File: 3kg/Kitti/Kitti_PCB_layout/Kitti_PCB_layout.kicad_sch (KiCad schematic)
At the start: 39 parts, among them IC1 TEENSY_4.1, J1 JS17250, J10 Omron E3Z-D82, J11 Omron E3Z-D82, J12 Omron E3Z-D82, J13 Omron E3Z-D82, J14 Omron E3Z-D82, J15 Omron E3Z-D82, J16 Omron E3Z-D82, J17 Omron E3Z-D82, J18 Conn_02x05_Odd_Even, J19 Conn_01x03_Pin, J2 JS17250, J3 JS17250, J4 JS17250, J5 TF_mini, J6 TF_mini, J7 TF_mini, J8 TF_mini, J9 Omron E3Z-D82, U1 AMS1117-5.0

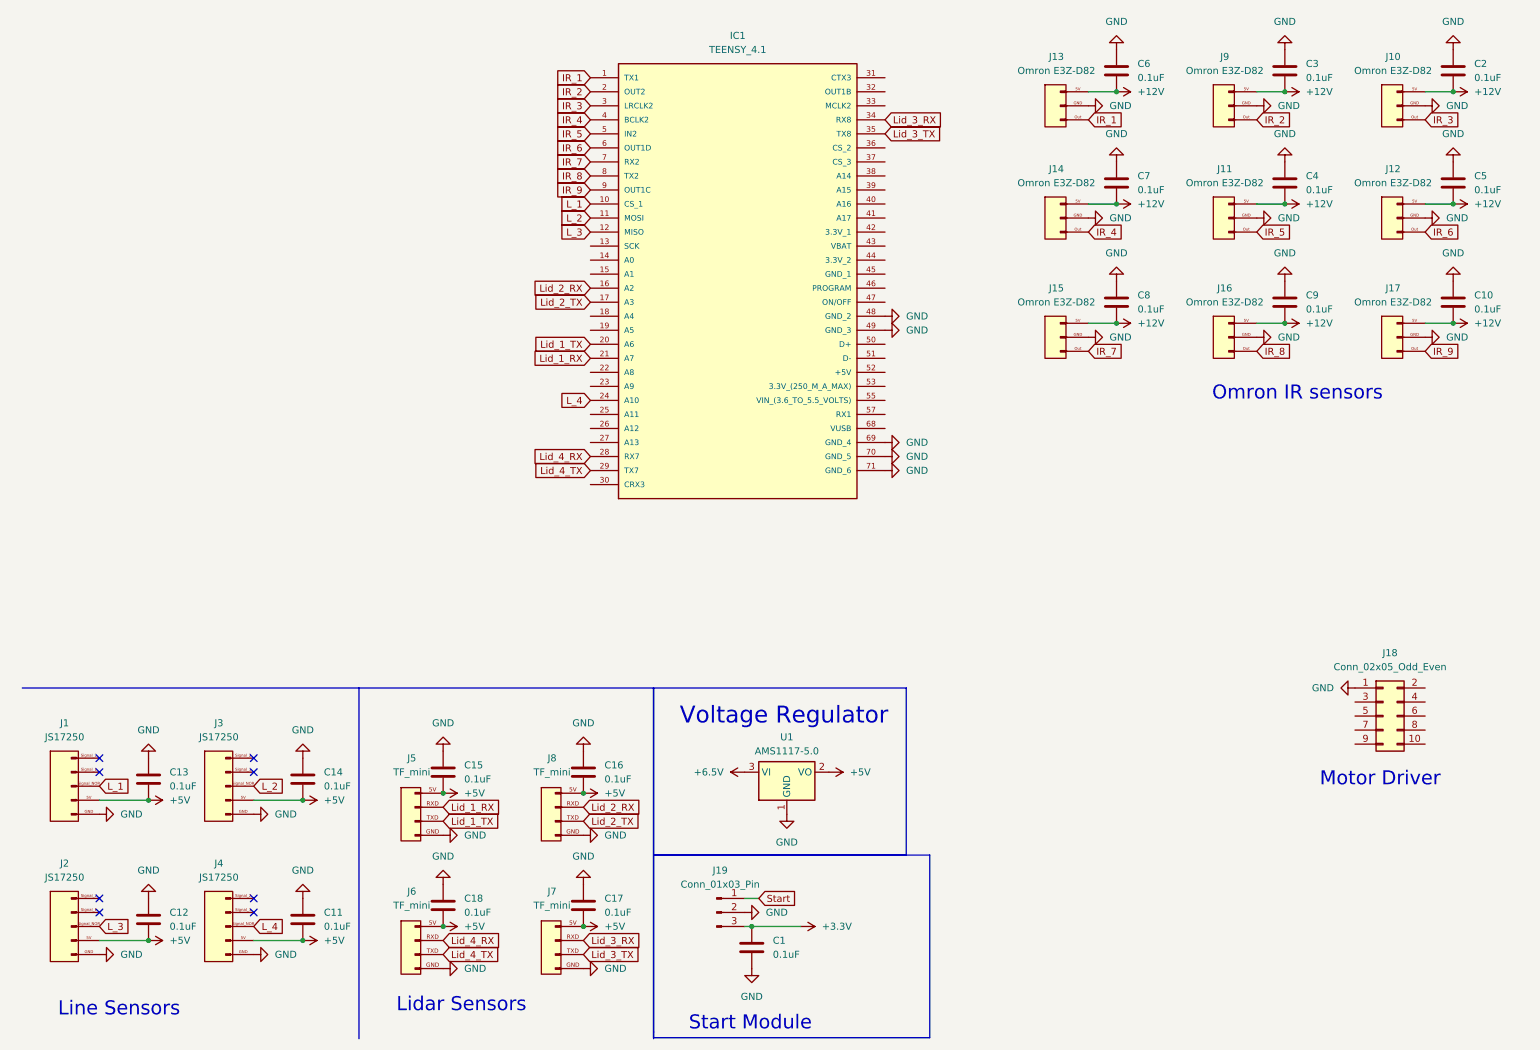
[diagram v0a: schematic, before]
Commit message: resistor and motor driver
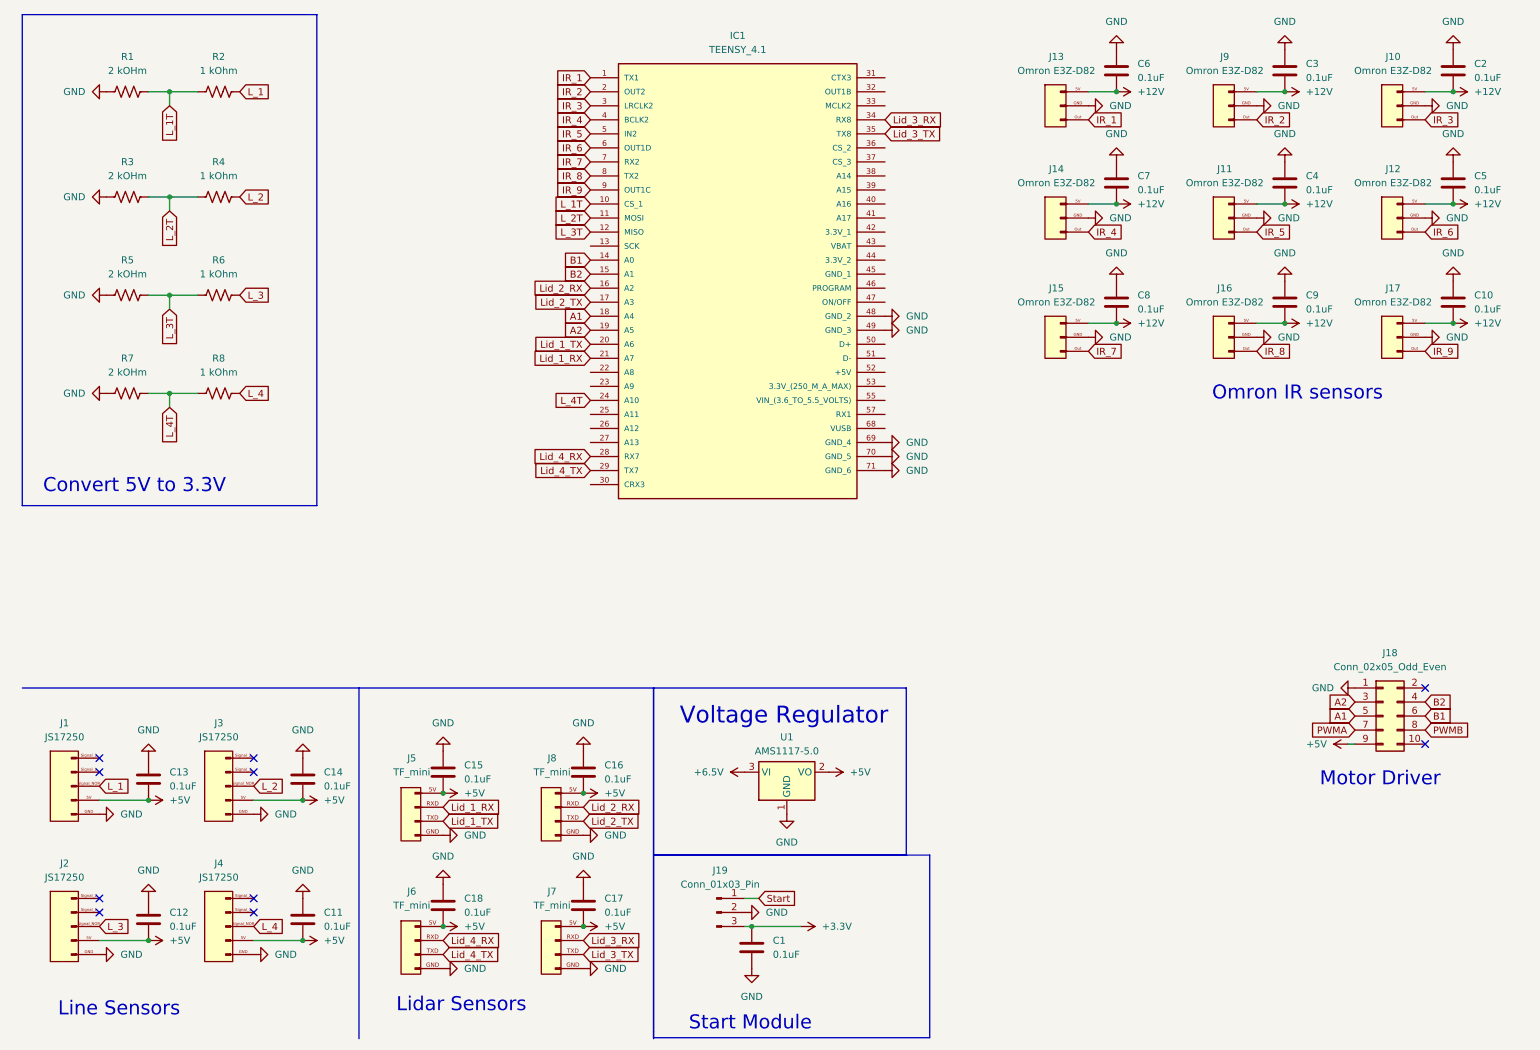
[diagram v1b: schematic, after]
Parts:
- added R1, R3, R5, R7: 2 kOHm, symbol Device:R_US
- added R2, R4, R6, R8: 1 kOhm, symbol Device:R_US
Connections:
- net +5V: now also J18.9 (Pin_9)
- net GND: now also R1.1, R3.1, R5.1, R7.1
- net L_1: now also R2.2; no longer IC1.10 (CS_1)
- net L_2: now also R4.2; no longer IC1.11 (MOSI)
- net L_3: now also R6.2; no longer IC1.12 (MISO)
- net L_4: now also R8.2; no longer IC1.24 (A10)
- net A2: now reaches J18.3 (Pin_3)
- net A2: now also IC1.19 (A5)
- net B2: now reaches J18.4 (Pin_4)
- net B2: now also IC1.15 (A1)
- net A1: now reaches J18.5 (Pin_5)
- net A1: now also IC1.18 (A4)
- net B1: now reaches J18.6 (Pin_6)
- net B1: now also IC1.14 (A0)
- net PWMA: now reaches J18.7 (Pin_7)
- net PWMB: now reaches J18.8 (Pin_8)
- new net L_1T: IC1.10 (CS_1), R1.2, R2.1
- new net L_2T: IC1.11 (MOSI), R3.2, R4.1
- new net L_3T: IC1.12 (MISO), R5.2, R6.1
- new net L_4T: IC1.24 (A10), R7.2, R8.1
- no-connect marks 8 -> 10
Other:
- note added: "Convert 5V to 3.3V"

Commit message: kitti
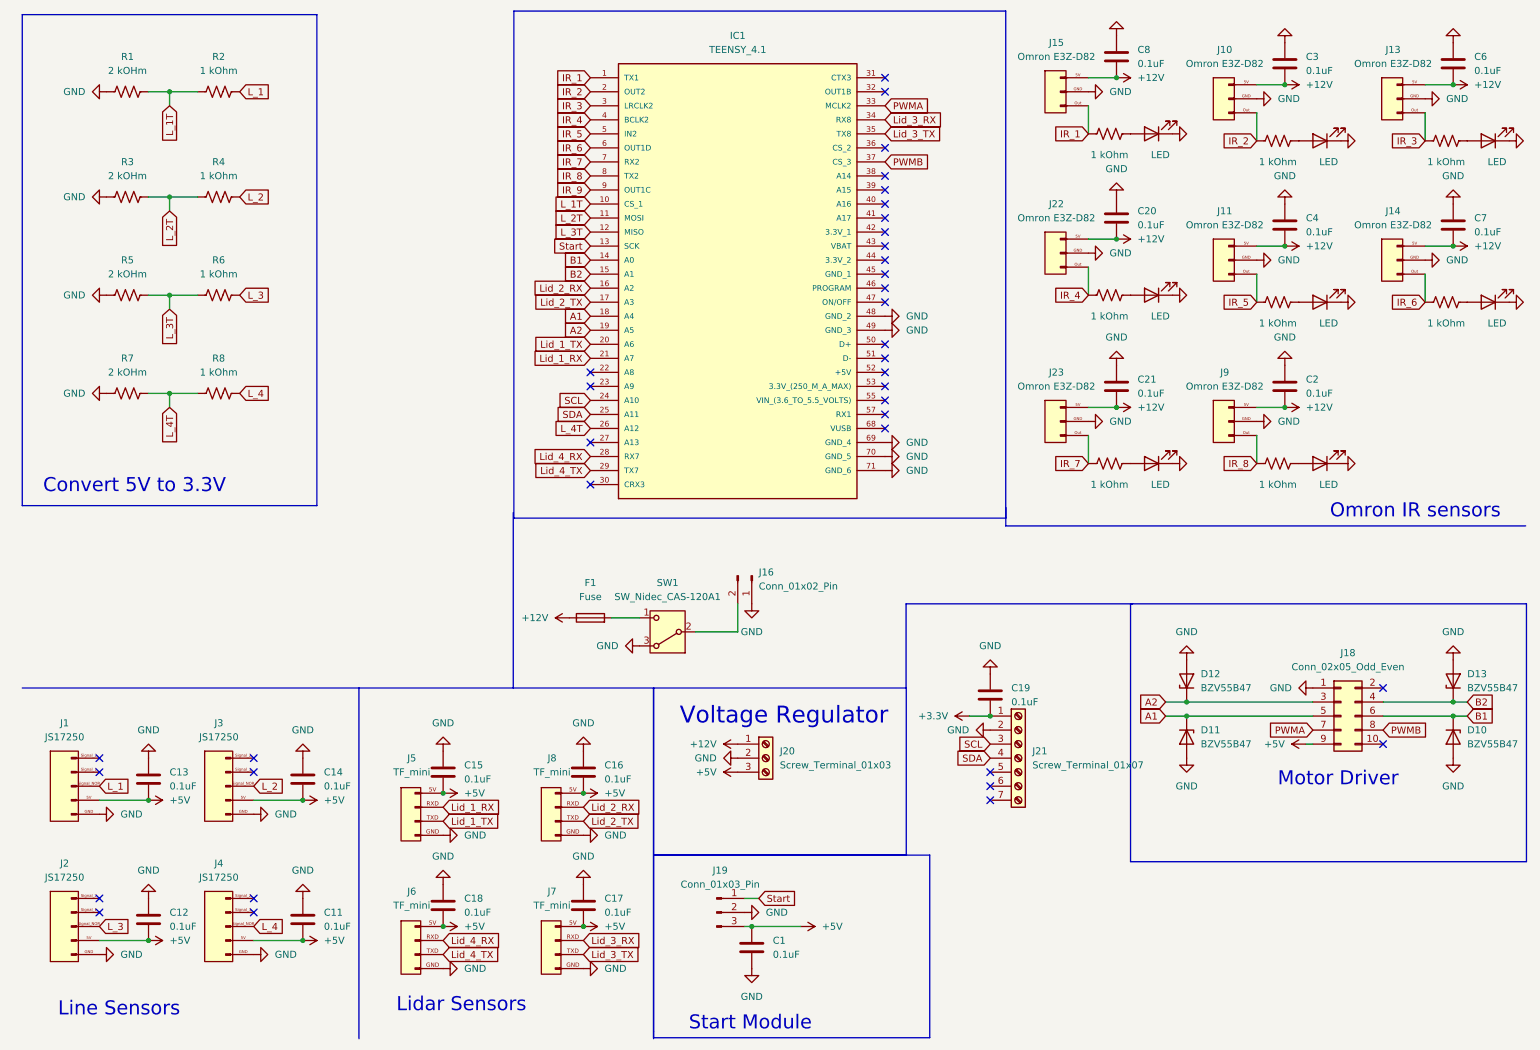
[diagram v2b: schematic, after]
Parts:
- removed C10, C5, C9: 0.1uF, symbol Device:C
- removed J12, J16, J17: Omron E3Z-D82, symbol IRsensor:Omron E3Z-D82
- removed U1: AMS1117-5.0, Package_TO_SOT_SMD:SOT-223-3_TabPin2, symbol Regulator_Linear:AMS1117-5.0
- added C19, C20, C21: 0.1uF, Capacitor_SMD:C_0805_2012Metric_Pad1.18x1.45mm_HandSolder, symbol Device:C
- added D1, D2, D3, D4, D5, D7, D8, D9: LED, LED_SMD:LED_1206_3216Metric_Pad1.42x1.75mm_HandSolder, symbol Device:LED
- added D10, D11, D12, D13: BZV55B47, Diode_SMD:D_MiniMELF, symbol Diode:BZV55B47
- added F1: Fuse, Fuse:Fuse_0805_2012Metric_Pad1.15x1.40mm_HandSolder, symbol Device:Fuse
- added J16: Conn_01x02_Pin, TerminalBlock_TE-Connectivity:TerminalBlock_TE_282834-2_1x02_P2.54mm_Horizontal, symbol Connector:Conn_01x02_Pin
- added J20: Screw_Terminal_01x03, TerminalBlock_TE-Connectivity:TerminalBlock_TE_282834-3_1x03_P2.54mm_Horizontal, symbol Connector:Screw_Terminal_01x03
- added J21: Screw_Terminal_01x07, TerminalBlock_TE-Connectivity:TerminalBlock_TE_282834-7_1x07_P2.54mm_Horizontal, symbol Connector:Screw_Terminal_01x07
- added J22, J23: Omron E3Z-D82, TerminalBlock_TE-Connectivity:TerminalBlock_TE_282834-3_1x03_P2.54mm_Horizontal, symbol IRsensor:Omron E3Z-D82
- added R10, R11, R12, R13, R15, R16, R17, R9: 1 kOhm, Resistor_SMD:R_0805_2012Metric_Pad1.20x1.40mm_HandSolder, symbol Device:R_US
- added SW1: SW_Nidec_CAS-120A1, Button_Switch_SMD:Nidec_Copal_CAS-120A, symbol Switch:SW_Nidec_CAS-120A1
- C1, C11, C12, C13, C14, C15, C16, C17, C18, C2, C3, C4, C6, C7, C8: footprint (none) -> Capacitor_SMD:C_0805_2012Metric_Pad1.18x1.45mm_HandSolder
- J1, J10, J11, J13, J14, J15, J19, J2, J3, J4, J9: footprint (none) -> TerminalBlock_TE-Connectivity:TerminalBlock_TE_282834-3_1x03_P2.54mm_Horizontal
- J18: footprint (none) -> Connector_PinHeader_2.54mm:PinHeader_2x05_P2.54mm_Horizontal
- J5, J6, J7, J8: footprint (none) -> TerminalBlock_TE-Connectivity:TerminalBlock_TE_282834-4_1x04_P2.54mm_Horizontal
- R1, R2, R3, R4, R5, R6, R7, R8: footprint (none) -> Resistor_SMD:R_0805_2012Metric_Pad1.20x1.40mm_HandSolder
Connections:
- net +12V: now also C20.2, C21.2, F1.1, J20.1 (Pin_1), J22.5V (Pin_1), J23.5V (Pin_1)
- net +3.3V: now also C19.2, J21.1 (Pin_1); no longer C1.1, J19.3 (Pin_3)
- net +5V: now also C1.1, J19.3 (Pin_3), J20.3 (Pin_3)
- net A1: now also D11.1 (K)
- net A2: now also D12.1 (K)
- net B1: now also D10.1 (K)
- net B2: now also D13.1 (K)
- net GND: now also C19.1, C20.1, C21.1, D1.1 (K), D10.2 (A), D11.2 (A), D12.2 (A), D13.2 (A), D2.1 (K), D3.1 (K), D4.1 (K), D5.1 (K), D7.1 (K), D8.1 (K), D9.1 (K), J16.1 (Pin_1), J20.2 (Pin_2), J21.2 (Pin_2), J22.GND (Pin_2), J23.GND (Pin_2), SW1.3 (A)
- net IR_1: now also J15.Out (Pin_3), R15.2; no longer J13.Out (Pin_3)
- net IR_2: now also J10.Out (Pin_3), R12.2; no longer J9.Out (Pin_3)
- net IR_3: now also J13.Out (Pin_3), R16.2; no longer J10.Out (Pin_3)
- net IR_4: now also J22.Out (Pin_3), R9.2; no longer J14.Out (Pin_3)
- net IR_5: now also R13.2
- net IR_6: now also J14.Out (Pin_3), R17.2
- net IR_7: now also J23.Out (Pin_3), R10.2; no longer J15.Out (Pin_3)
- net IR_8: now also J9.Out (Pin_3), R11.2
- net L_4T: now also IC1.26 (A12); no longer IC1.24 (A10)
- net PWMA: now also IC1.33 (MCLK2)
- net PWMB: now also IC1.37 (CS_3)
- net Start: now also IC1.13 (SCK)
- net SDA: now reaches IC1.25 (A11)
- net SDA: now also J21.4 (Pin_4)
- new net: D4.2 (A), R12.1
- new net: D3.2 (A), R11.1
- new net: D9.2 (A), R17.1
- new net: D7.2 (A), R15.1
- new net: D2.2 (A), R10.1
- new net: D1.2 (A), R9.1
- new net: D8.2 (A), R16.1
- new net: J16.2 (Pin_2), SW1.2 (B)
- new net: F1.2, SW1.1 (C)
- new net: D5.2 (A), R13.1
- new net SCL: IC1.24 (A10), J21.3 (Pin_3)
- no-connect marks 10 -> 37
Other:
- moved on the sheet: C8, J15, J18

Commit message: Kitti to Strawberri
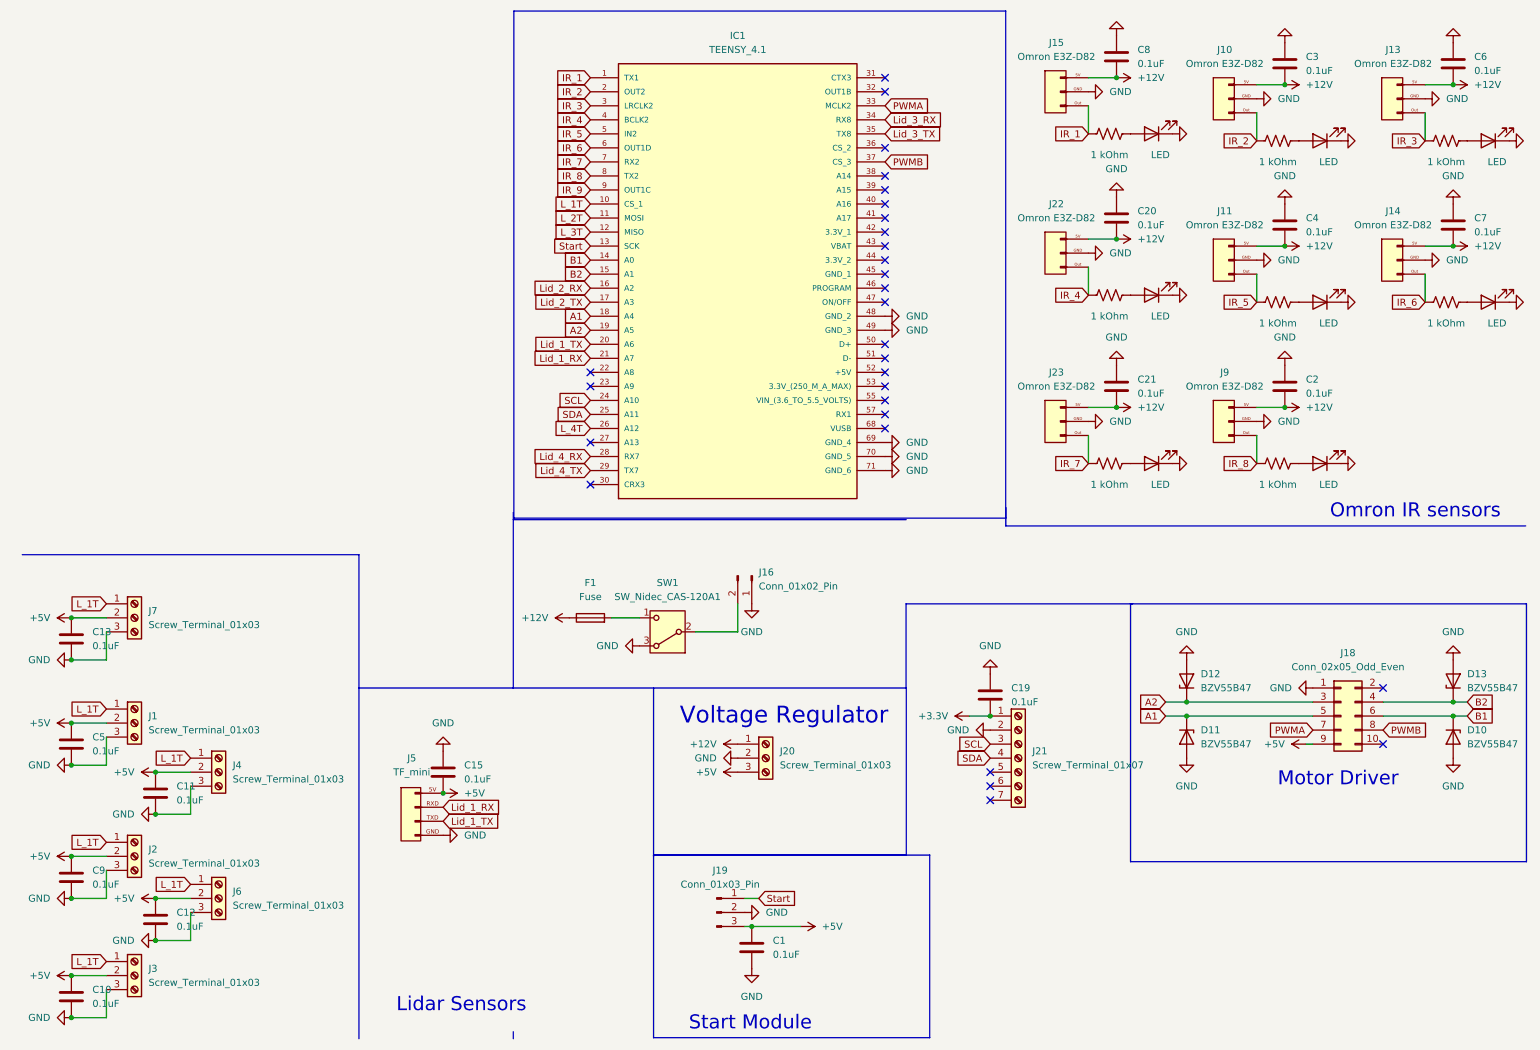
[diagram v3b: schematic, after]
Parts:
- removed C14, C16, C17, C18: 0.1uF, Capacitor_SMD:C_0805_2012Metric_Pad1.18x1.45mm_HandSolder, symbol Device:C
- removed J1, J2, J3, J4: JS17250, TerminalBlock_TE-Connectivity:TerminalBlock_TE_282834-3_1x03_P2.54mm_Horizontal, symbol Line_Sensors:JS17250
- removed J6, J7, J8: TF_mini, TerminalBlock_TE-Connectivity:TerminalBlock_TE_282834-4_1x04_P2.54mm_Horizontal, symbol LidarSensor:TF_mini
- removed R1, R3, R5, R7: 2 kOHm, Resistor_SMD:R_0805_2012Metric_Pad1.20x1.40mm_HandSolder, symbol Device:R_US
- removed R2, R4, R6, R8: 1 kOhm, Resistor_SMD:R_0805_2012Metric_Pad1.20x1.40mm_HandSolder, symbol Device:R_US
- added C10, C5, C9: 0.1uF, symbol Device:C
- added J1, J2, J3, J4, J6, J7: Screw_Terminal_01x03, TerminalBlock_TE-Connectivity:TerminalBlock_TE_282834-3_1x03_P2.54mm_Horizontal, symbol Connector:Screw_Terminal_01x03
- C11, C12, C13: footprint Capacitor_SMD:C_0805_2012Metric_Pad1.18x1.45mm_HandSolder -> (none)
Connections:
- net +5V: now also C11.1, C12.1, C13.1, C10.1, C5.1, C9.1, J1.2 (Pin_2), J2.2 (Pin_2), J3.2 (Pin_2), J4.2 (Pin_2), J6.2 (Pin_2), J7.2 (Pin_2); no longer C11.2, C12.2, C13.2
- net GND: now also C11.2, C12.2, C13.2, C10.2, C5.2, C9.2, J1.3 (Pin_3), J2.3 (Pin_3), J3.3 (Pin_3), J4.3 (Pin_3), J6.3 (Pin_3), J7.3 (Pin_3); no longer C11.1, C12.1, C13.1
- net L_1T: now also J1.1 (Pin_1), J2.1 (Pin_1), J3.1 (Pin_1), J4.1 (Pin_1), J6.1 (Pin_1), J7.1 (Pin_1)
- no-connect marks 37 -> 29
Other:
- note removed: "Convert 5V to 3.3V"
- note removed: "Line Sensors"
